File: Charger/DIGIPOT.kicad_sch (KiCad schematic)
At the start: 0 parts

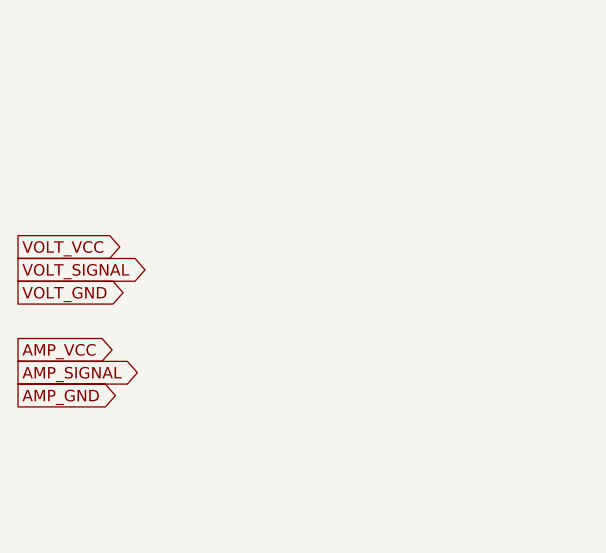
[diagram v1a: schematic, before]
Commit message: Charger WIP
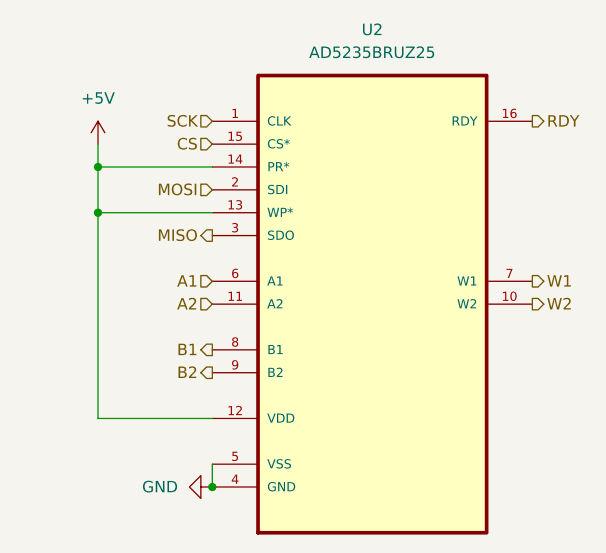
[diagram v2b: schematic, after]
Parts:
- added U2: AD5235BRUZ25, AD5235BRUZ25:SOP65P640X120-16N, symbol AD5235BRUZ25:AD5235BRUZ25
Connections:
- new net +5V: U2.12 (VDD), U2.13 (WP*), U2.14 (PR*)
- new net A1: U2.6 (A1)
- new net A2: U2.11 (A2)
- new net B1: U2.8 (B1)
- new net B2: U2.9 (B2)
- new net CS: U2.15 (CS*)
- new net GND: U2.4 (GND), U2.5 (VSS)
- new net MISO: U2.3 (SDO)
- new net MOSI: U2.2 (SDI)
- new net RDY: U2.16 (RDY)
- new net SCK: U2.1 (CLK)
- new net W1: U2.7 (W1)
- new net W2: U2.10 (W2)
